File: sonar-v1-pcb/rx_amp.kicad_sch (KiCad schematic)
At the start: 13 parts, among them U301 Opamp_Dual

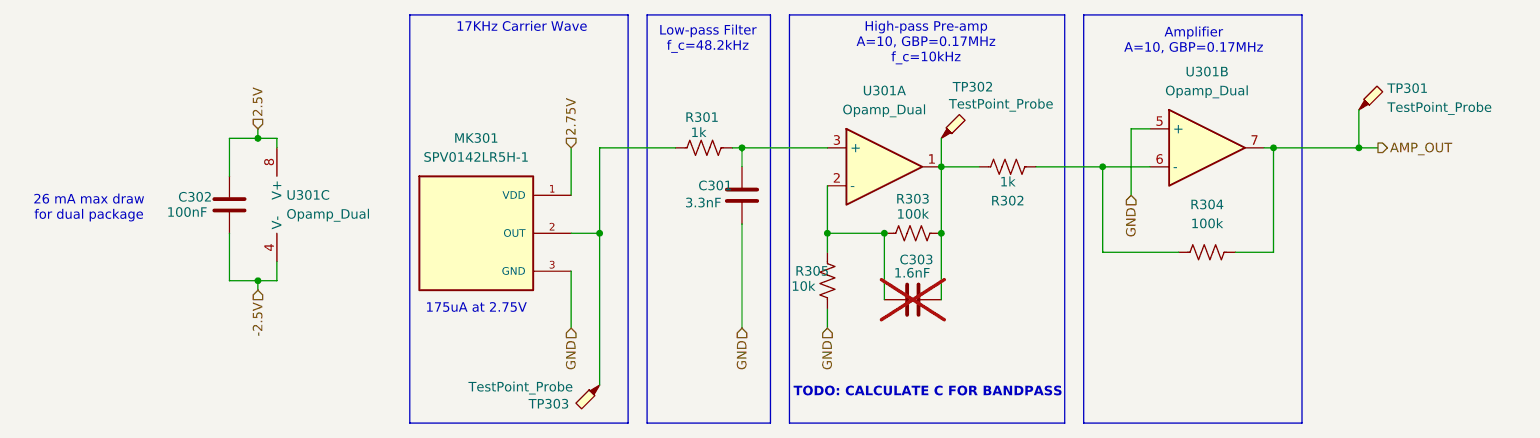
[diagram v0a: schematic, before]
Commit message: formatting lol
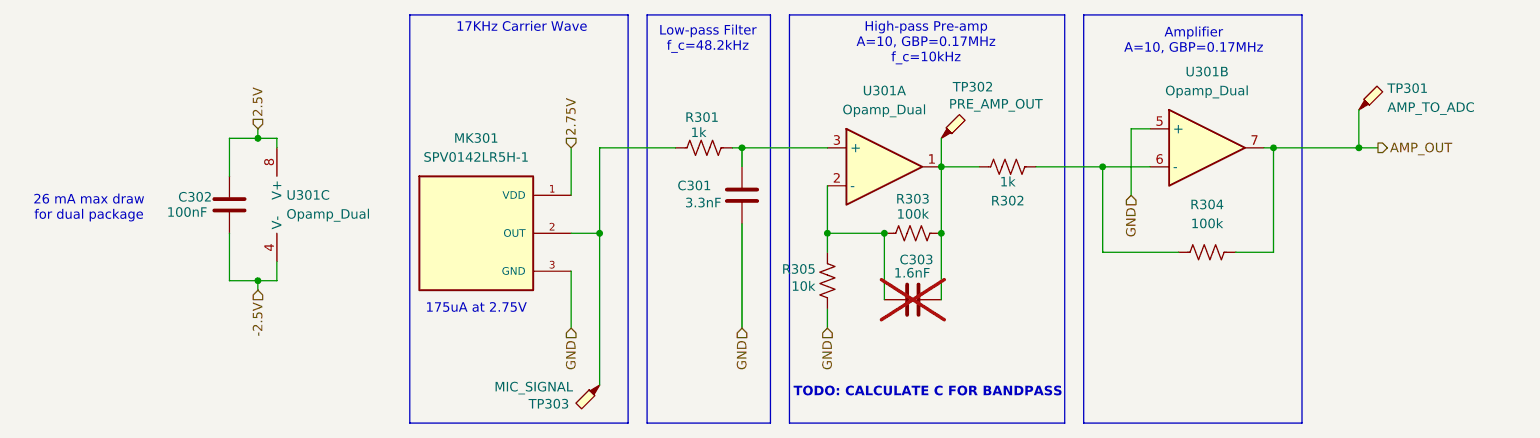
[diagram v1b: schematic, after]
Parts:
- TP301: value TestPoint_Probe -> AMP_TO_ADC
- TP302: value TestPoint_Probe -> PRE_AMP_OUT
- TP303: value TestPoint_Probe -> MIC_SIGNAL
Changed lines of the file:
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@@
 			)
 		)
-		(property "Value" "TestPoint_Probe"
+		(property "Value" "MIC_SIGNAL"
 			(at 113.284 108.204 0)
 			(effects
@@
 		(dnp no)
 		(property "Reference" "R305"
-			(at 143.002 92.71 0)
+			(at 141.224 92.456 0)
 			(effects
 				(font
@@
 			)
 		)
-		(property "Value" "TestPoint_Probe"
+		(property "Value" "PRE_AMP_OUT"
 			(at 163.576 70.358 0)
 			(effects
@@
 		(dnp no)
 		(property "Reference" "C301"
-			(at 130.048 81.28 0)
+			(at 127.254 81.28 0)
 			(effects
 				(font
@@
 			)
 		)
-		(property "Value" "TestPoint_Probe"
+		(property "Value" "AMP_TO_ADC"
 			(at 222.25 70.8024 0)
 			(effects
